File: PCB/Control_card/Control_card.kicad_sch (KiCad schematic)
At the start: 27 parts, among them IC1 TLSR8253F512ET48, J1 Conn_02x04_Counter_Clockwise, Y1 Crystal_GND24

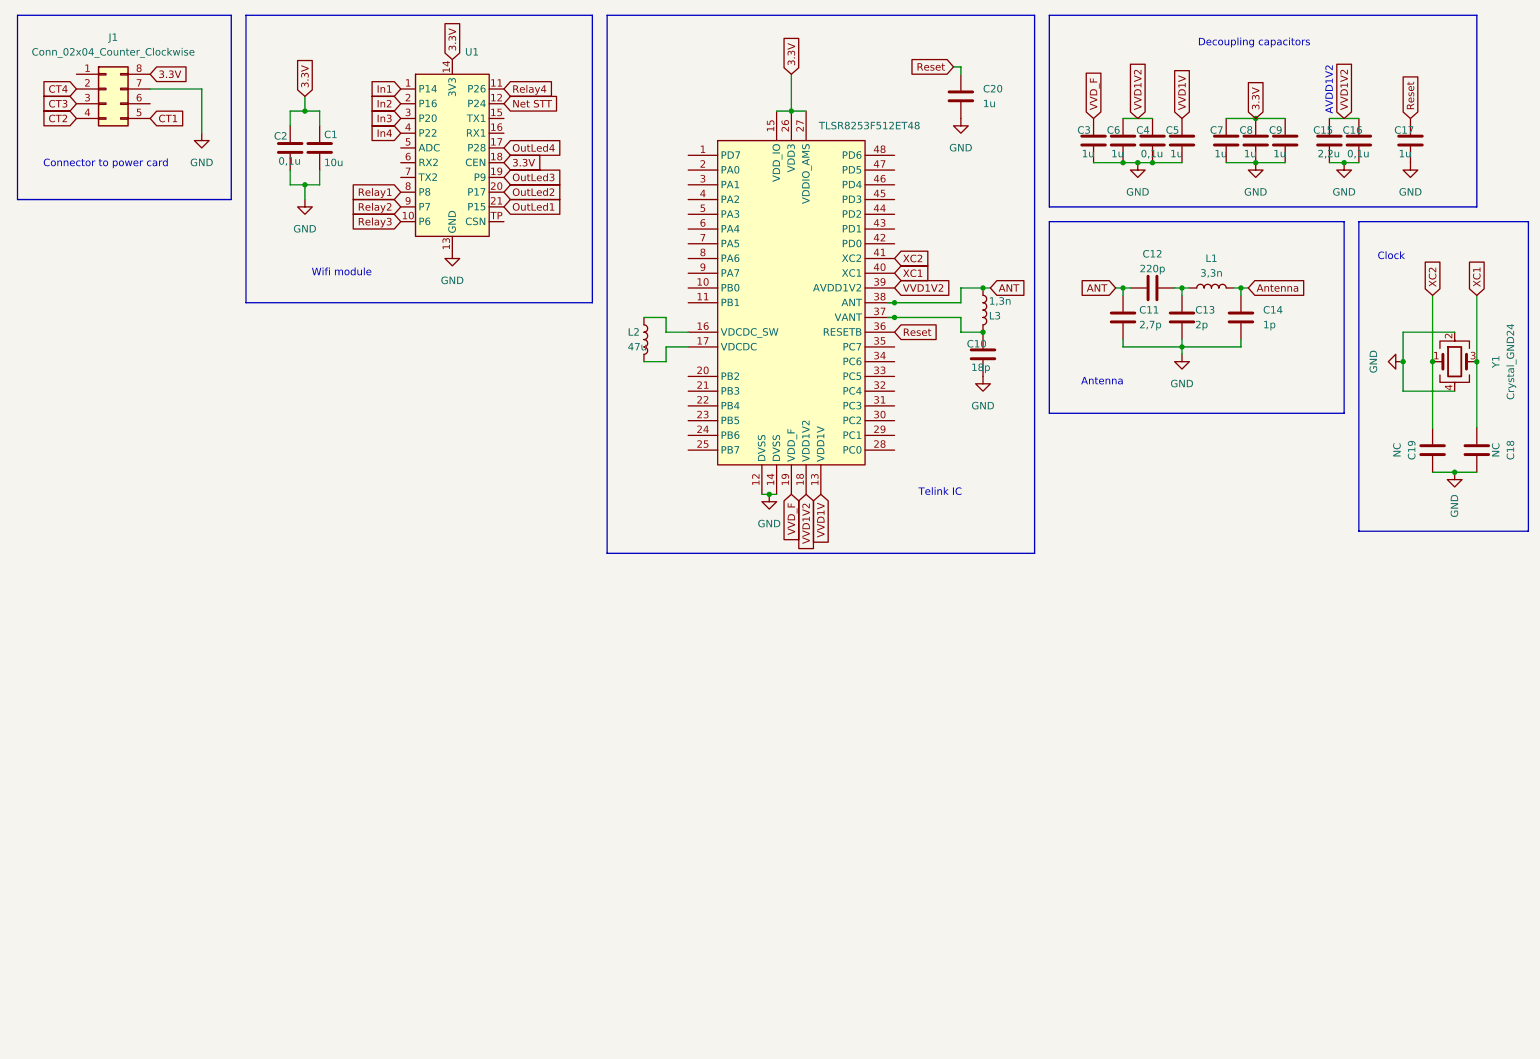
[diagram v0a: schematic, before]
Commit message: Ajout crystal
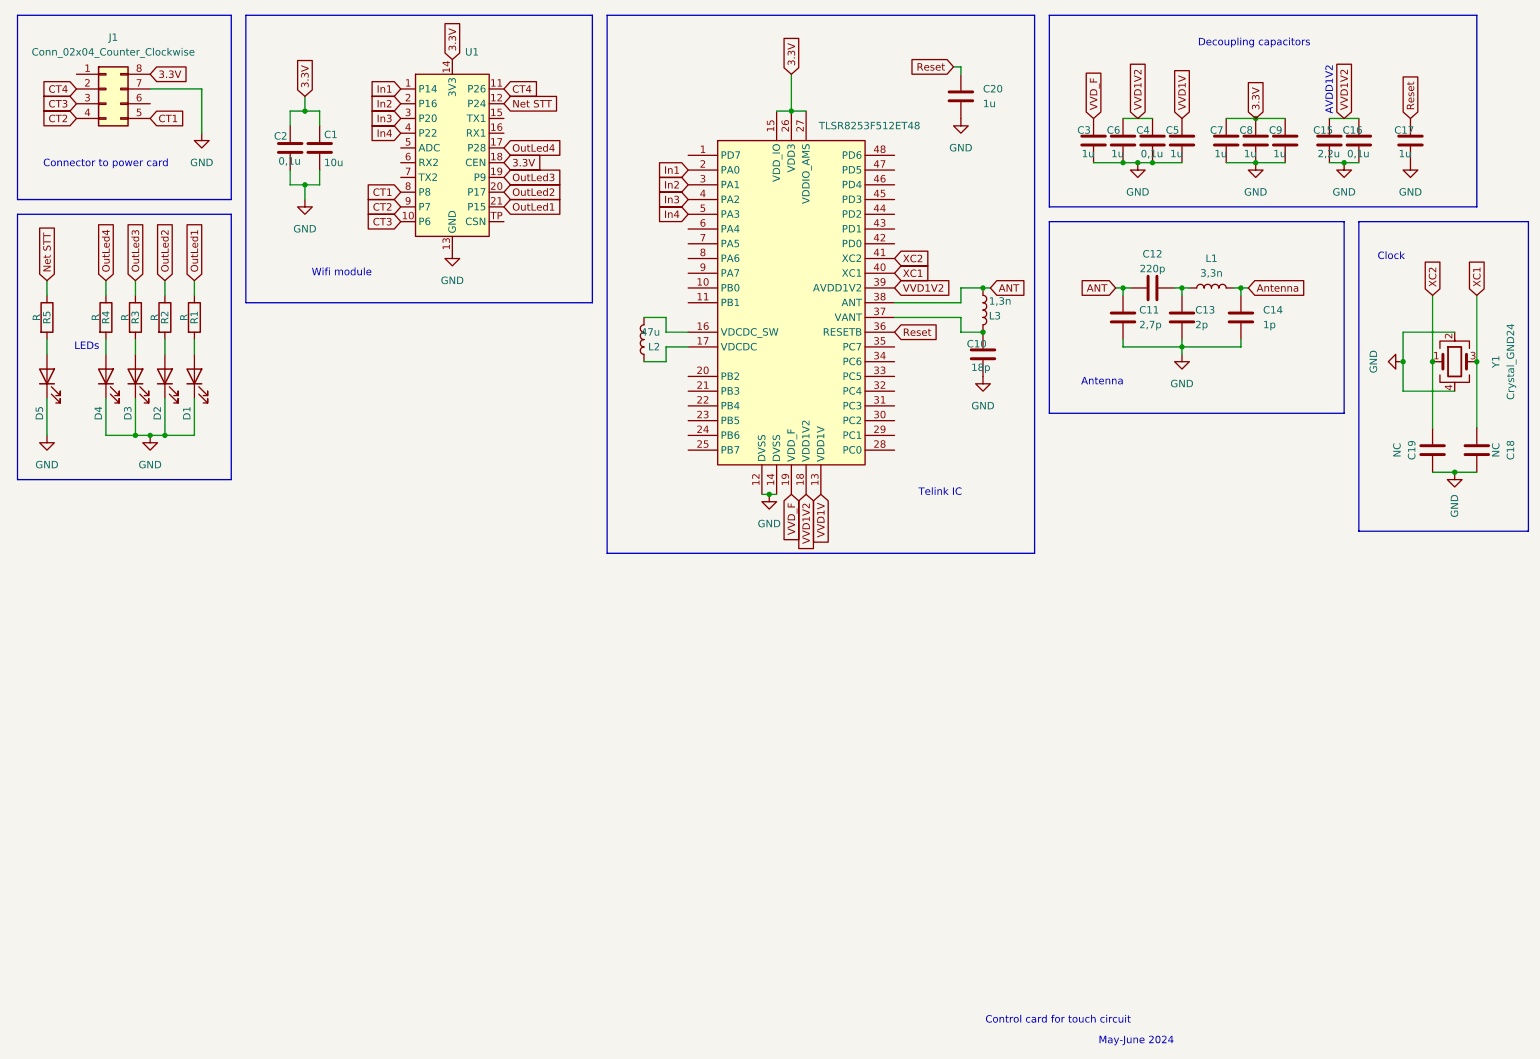
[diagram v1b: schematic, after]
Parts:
- added D1, D2, D3, D4, D5: LED, symbol Device:LED
- added R1, R2, R3, R4, R5: R, symbol Device:R
- U1: footprint (none) -> Touch_Switch_Custom:BK7231N
- Y1: footprint (none) -> Touch_Switch_Custom:Crystal
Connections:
- net Relay1 is gone; now on net CT1: U1.8 (P8)
- net Relay2 is gone; now on net CT2: U1.9 (P7)
- net Relay3 is gone; now on net CT3: U1.10 (P6)
- net Relay4 is gone; now on net CT4: U1.11 (P26)
- net GND: now also D1.1 (K), D2.1 (K), D3.1 (K), D4.1 (K), D5.1 (K)
- net In1: now also IC1.2 (PA0)
- net In2: now also IC1.3 (PA1)
- net In3: now also IC1.4 (PA2)
- net In4: now also IC1.5 (PA3)
- net Net STT: now also R5.1
- net OutLed1: now also R1.1
- net OutLed2: now also R2.1
- net OutLed3: now also R3.1
- net OutLed4: now also R4.1
- net at L2.1: now also IC1.17 (VDCDC); no longer IC1.16 (VDCDC_SW)
- net at L2.2: now also IC1.16 (VDCDC_SW); no longer IC1.17 (VDCDC)
- new net: D2.2 (A), R2.2
- new net: D4.2 (A), R4.2
- new net: D1.2 (A), R1.2
- new net: D3.2 (A), R3.2
- new net: D5.2 (A), R5.2
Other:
- note added: "Control card for touch circuit"
- note added: "LEDs"
- note added: "May-June 2024"
- moved on the sheet: L2
